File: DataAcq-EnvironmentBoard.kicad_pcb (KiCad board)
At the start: 2 copper layers, 42 x 50.2 mm, 22 parts, among them J1 CAN Output, J2 CAN Input, U1 SHT45, U2 FS3000-1005, U3 LMT87DCK, U4 Daughterboard Connector

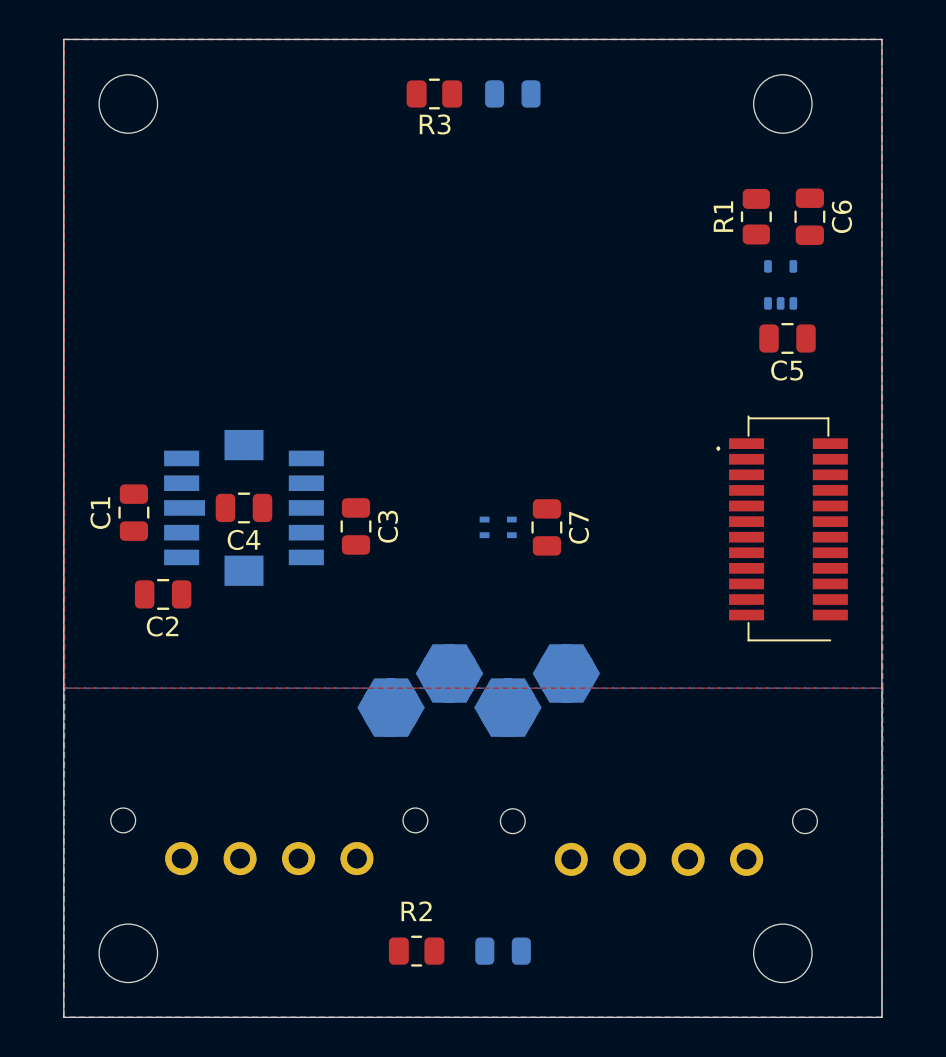
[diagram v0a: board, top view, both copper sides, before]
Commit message: routing
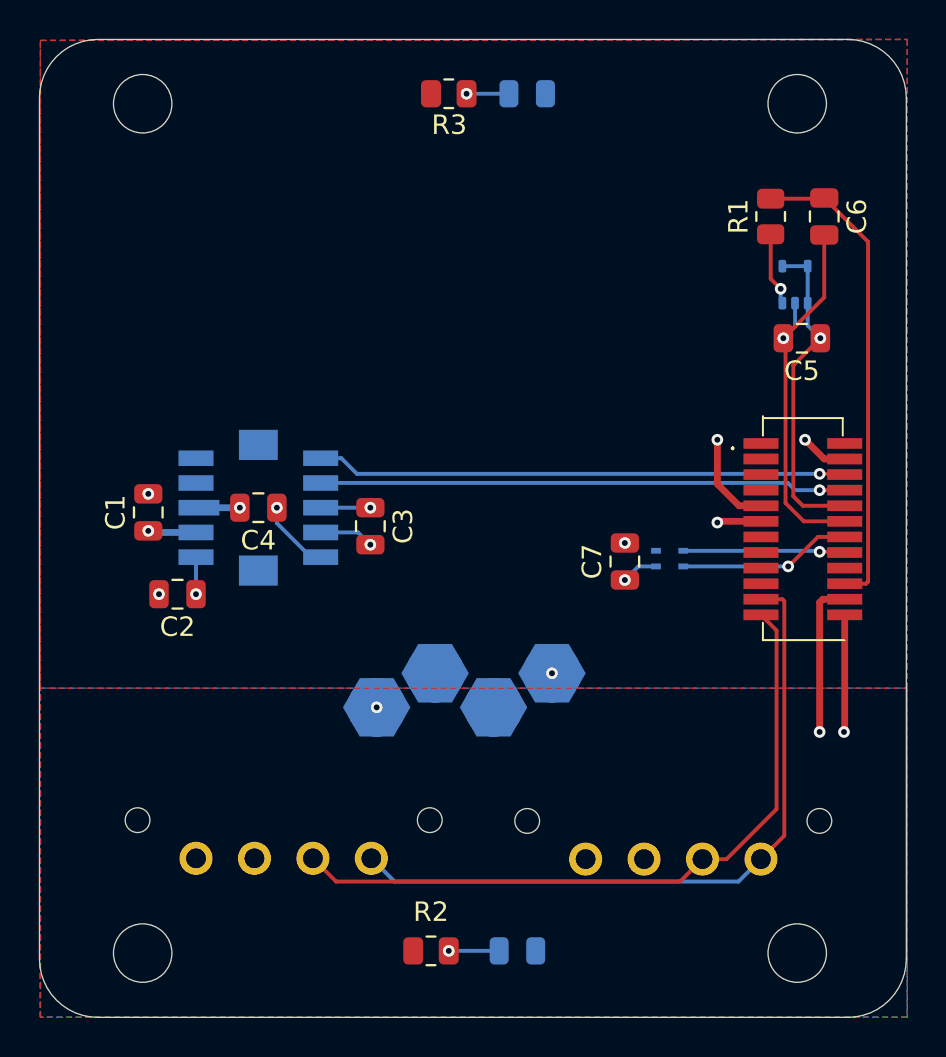
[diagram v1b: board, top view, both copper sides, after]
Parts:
- moved U1 8.94 mm to (172.3, 97.8), turned to 180 degrees
- moved C7 4.37 mm to (170.0, 98.0), turned to 90 degrees
- moved TP1 0.74 mm to (157.3, 105.5)
- moved TP2 0.74 mm to (163.3, 105.5)
- moved TP4 0.74 mm to (166.3, 103.7)
- moved TP5 0.74 mm to (160.3, 103.7)
- moved C3 0.74 mm to (156.9, 96.2)
- moved C4 0.74 mm to (151.2, 95.2)
- moved U2 0.74 mm to (151.2, 95.2)
- moved U4 0.74 mm to (160.8, 93.1)
- moved J1 0.74 mm to (177.0, 113.3)
- moved C1 0.74 mm to (145.5, 95.5)
- moved C2 0.74 mm to (147.0, 99.7)
- moved C5 0.74 mm to (179.1, 86.5)
- moved C6 0.74 mm to (180.2, 80.3)
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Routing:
- net /CAN_H: track 0.00 -> 36.1 mm
- net /CAN_L: track 0.00 -> 35.9 mm
- net /I2C2_SDA: track 0.00 -> 27.2 mm, vias 0 -> 1
- net /I2C2_SCL: track 0.00 -> 27.1 mm, vias 0 -> 1
- net /PA1(ADC): track 0.00 -> 24.6 mm
- net GNDA: track 0.00 -> 20.2 mm, vias 0 -> 1
- net VDDA: track 0.00 -> 16.8 mm, vias 0 -> 1
- net +3.3V: track 0.00 -> 9.35 mm, vias 0 -> 4
- net /I2C1_SCL: track 0.00 -> 8.91 mm, vias 0 -> 1
- net /I2C1_SDA: track 0.00 -> 8.32 mm, vias 0 -> 1
- net +12V_In: track 0.00 -> 8.02 mm, vias 0 -> 2
- net GND: track 0.00 -> 6.81 mm, vias 0 -> 6
- net GNDPWR: track 0.00 -> 6.03 mm, vias 0 -> 1
- net /TEMP_OUT: track 0.00 -> 3.79 mm, vias 0 -> 1
- net /AFLW_VCM: track 0.00 -> 3.76 mm, vias 0 -> 1
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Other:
- board size 42 x 50.2 mm -> 44.5 x 50.2 mm
